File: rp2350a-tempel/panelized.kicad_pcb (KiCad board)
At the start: 2 copper layers, 119.4 x 128.7 mm, 333 parts, among them J1 Conn_North, J2 Conn_East, J3 Conn_South, J4 Conn_West, SW1 BOOT SELECTOR, SW2 RST, U1 AMS1117-3.3, U2 W25Q16JVSS, U3 RP2350_60QFN, Y1 12Mhz HC49-SD

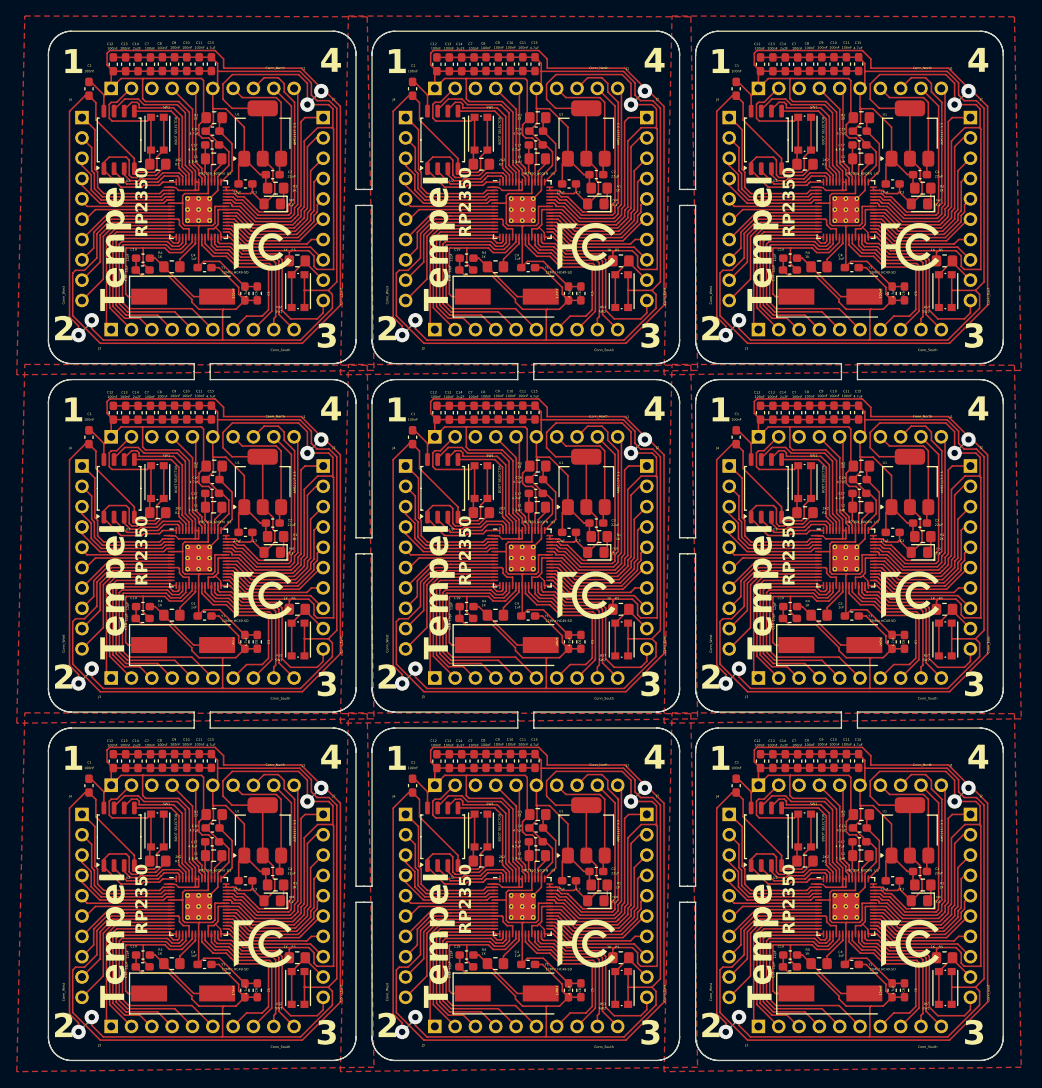
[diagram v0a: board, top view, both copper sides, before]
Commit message: chore: update after first prototype created
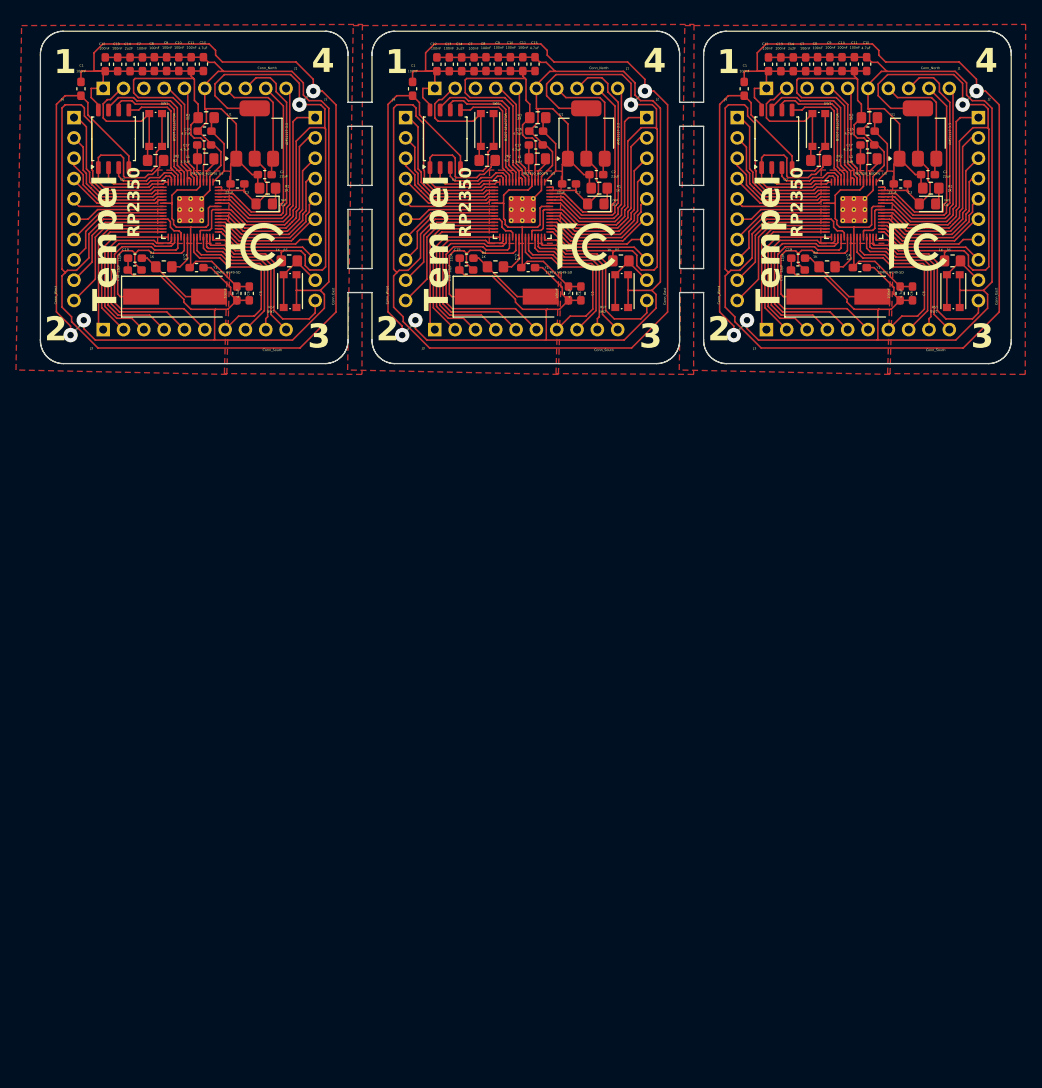
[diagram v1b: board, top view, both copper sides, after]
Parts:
- removed the C1 at (134.3, 70.8)
- removed the C1 at (93.9, 70.8)
- removed the C1 at (174.8, 70.8)
- removed the C1 at (134.3, 114.3)
- removed the C1 at (174.8, 27.2)
- removed the C1 at (93.9, 114.3)
- removed the C1 at (174.8, 114.3)
- removed the C1 at (93.9, 27.2)
- removed the C10 at (187.0, 67.7)
- removed the C10 at (146.6, 111.2)
- removed the C10 at (106.1, 111.2)
- removed the C10 at (146.6, 67.7)
- removed the C10 at (187.0, 111.2)
- removed the C10 at (106.1, 67.7)
- removed the C10 at (106.1, 24.1)
- removed the C10 at (187.0, 24.1)
- removed the C11 at (107.7, 111.2)
- removed the C11 at (188.6, 67.7)
- removed the C11 at (148.1, 111.2)
- removed the C11 at (107.7, 67.7)
- removed the C11 at (188.6, 111.2)
- removed the C11 at (107.7, 24.1)
- removed the C11 at (188.6, 24.1)
- removed the C11 at (148.1, 67.7)
- removed the C12 at (96.9, 111.2)
- removed the C12 at (137.4, 111.2)
- removed the C12 at (96.9, 67.7)
- removed the C12 at (177.8, 24.1)
- removed the C12 at (96.9, 24.1)
- removed the C12 at (177.8, 111.2)
- removed the C12 at (177.8, 67.7)
- removed the C12 at (137.4, 67.7)
- removed the C13 at (138.9, 67.7)
- removed the C13 at (179.4, 67.7)
- removed the C13 at (138.9, 111.2)
- removed the C13 at (98.5, 24.1)
- removed the C13 at (179.4, 111.2)
- removed the C13 at (98.5, 111.2)
- removed the C13 at (179.4, 24.1)
- removed the C13 at (98.5, 67.7)
- removed the C14 at (180.9, 24.1)
- removed the C14 at (180.9, 67.7)
- removed the C14 at (180.9, 111.2)
- removed the C14 at (140.5, 111.2)
- removed the C14 at (100.0, 67.7)
- removed the C14 at (140.5, 67.7)
- removed the C14 at (100.0, 24.1)
- removed the C14 at (100.0, 111.2)
- removed the C15 at (109.2, 111.2)
- removed the C15 at (190.1, 111.2)
- removed the C15 at (109.2, 24.1)
- removed the C15 at (190.1, 67.7)
- removed the C15 at (109.2, 67.7)
- removed the C15 at (149.7, 67.7)
- removed the C15 at (190.1, 24.1)
- removed the C15 at (149.7, 111.2)
- removed the C16 at (109.3, 76.0)
- removed the C16 at (190.2, 32.5)
- removed the C16 at (149.8, 119.6)
- removed the C16 at (190.2, 76.0)
- removed the C16 at (149.8, 76.0)
- removed the C16 at (190.2, 119.6)
- removed the C16 at (109.3, 119.6)
- removed the C16 at (109.3, 32.5)
- removed the C17 at (109.3, 121.3)
- removed the C17 at (149.7, 121.3)
- removed the C17 at (190.2, 77.8)
- removed the C17 at (190.2, 121.3)
- removed the C17 at (109.3, 34.2)
- removed the C17 at (190.2, 34.2)
- removed the C17 at (149.7, 77.8)
- removed the C17 at (109.3, 77.8)
- removed the C18 at (100.6, 137.0)
- removed the C18 at (181.5, 49.8)
- removed the C18 at (181.5, 93.4)
- removed the C18 at (141.1, 93.4)
- removed the C18 at (141.1, 137.0)
- removed the C18 at (100.6, 49.8)
- removed the C18 at (100.6, 93.4)
- removed the C18 at (181.5, 137.0)
- removed the C19 at (141.1, 135.5)
- removed the C19 at (100.6, 91.9)
- removed the C19 at (181.5, 91.9)
- removed the C19 at (100.6, 135.5)
- removed the C19 at (141.1, 91.9)
- removed the C19 at (181.5, 48.4)
- removed the C19 at (181.5, 135.5)
- removed the C19 at (100.6, 48.4)
- removed the C2 at (197.8, 81.5)
- removed the C2 at (157.3, 125.0)
- removed the C2 at (116.9, 81.5)
- removed the C2 at (197.8, 37.9)
- removed the C2 at (197.8, 125.0)
- removed the C2 at (116.9, 125.0)
- removed the C2 at (116.9, 37.9)
- removed the C2 at (157.3, 81.5)
- removed the C3 at (113.5, 39.1)
- removed the C3 at (194.4, 39.1)
- removed the C3 at (113.5, 82.6)
- removed the C3 at (153.9, 82.6)
- removed the C3 at (113.5, 126.2)
- removed the C3 at (194.4, 126.2)
- removed the C3 at (194.4, 82.6)
- removed the C3 at (153.9, 126.2)
- removed the C4 at (189.2, 93.1)
- removed the C4 at (108.3, 136.7)
- removed the C4 at (189.2, 49.5)
- removed the C4 at (148.8, 93.1)
- removed the C4 at (108.3, 49.5)
- removed the C4 at (108.3, 93.1)
- removed the C4 at (189.2, 136.7)
- removed the C4 at (148.8, 136.7)
- removed the C5 at (195.8, 139.9)
- removed the C5 at (195.8, 52.8)
- removed the C5 at (114.9, 96.3)
- removed the C5 at (155.4, 96.3)
- removed the C5 at (114.9, 52.8)
- removed the C5 at (155.4, 139.9)
- removed the C5 at (195.8, 96.3)
- removed the C5 at (114.9, 139.9)
- removed the C6 at (153.8, 96.3)
- removed the C6 at (113.4, 139.9)
- removed the C6 at (194.3, 96.3)
- removed the C6 at (113.4, 52.8)
- removed the C6 at (194.3, 52.8)
- removed the C6 at (113.4, 96.3)
- removed the C6 at (194.3, 139.9)
- removed the C6 at (153.8, 139.9)
- removed the C7 at (182.5, 67.7)
- removed the C7 at (142.0, 67.7)
- removed the C7 at (101.6, 24.1)
- removed the C7 at (182.5, 111.2)
- removed the C7 at (101.6, 111.2)
- removed the C7 at (182.5, 24.1)
- removed the C7 at (101.6, 67.7)
- removed the C7 at (142.0, 111.2)
- removed the C8 at (184.0, 24.1)
- removed the C8 at (103.1, 111.2)
- removed the C8 at (103.1, 24.1)
- removed the C8 at (143.5, 67.7)
- removed the C8 at (184.0, 111.2)
- removed the C8 at (143.5, 111.2)
- removed the C8 at (103.1, 67.7)
- removed the C8 at (184.0, 67.7)
- removed the C9 at (145.1, 111.2)
- removed the C9 at (104.6, 111.2)
- removed the C9 at (185.5, 24.1)
- removed the C9 at (145.1, 67.7)
- removed the C9 at (185.5, 67.7)
- removed the C9 at (104.6, 24.1)
- removed the C9 at (104.6, 67.7)
- removed the C9 at (185.5, 111.2)
- removed the D1 at (116.8, 128.7)
- removed the D1 at (197.7, 128.7)
- removed the D1 at (116.8, 85.1)
- removed the D1 at (197.7, 41.6)
- removed the D1 at (157.3, 128.7)
- removed the D1 at (157.3, 85.1)
- removed the D1 at (197.7, 85.1)
- removed the D1 at (116.8, 41.6)
- removed the J1 at (96.7, 114.3)
- removed the J1 at (137.1, 70.7)
- removed the J1 at (177.6, 114.3)
- removed the J1 at (96.7, 27.1)
- removed the J1 at (177.6, 70.7)
- removed the J1 at (137.1, 114.3)
- removed the J1 at (177.6, 27.1)
- removed the J1 at (96.7, 70.7)
- removed the J2 at (163.6, 117.9)
- removed the J2 at (123.2, 30.8)
- removed the J2 at (163.6, 74.4)
- removed the J2 at (123.2, 117.9)
- removed the J2 at (204.1, 74.4)
- removed the J2 at (123.2, 74.4)
- removed the J2 at (204.1, 117.9)
- removed the J2 at (204.1, 30.8)
- removed the J3 at (96.7, 144.4)
- removed the J3 at (137.1, 100.9)
- removed the J3 at (177.6, 100.9)
- removed the J3 at (177.6, 144.4)
- removed the J3 at (177.6, 57.3)
- removed the J3 at (96.7, 57.3)
- removed the J3 at (96.7, 100.9)
- removed the J3 at (137.1, 144.4)
- removed the J4 at (93.0, 117.9)
- removed the J4 at (93.0, 74.4)
- removed the J4 at (133.5, 117.9)
- removed the J4 at (93.0, 30.8)
- removed the J4 at (173.9, 117.9)
- removed the J4 at (133.5, 74.4)
- removed the J4 at (173.9, 30.8)
- removed the J4 at (173.9, 74.4)
- removed the L1 at (109.5, 35.9)
- removed the L1 at (109.5, 123.1)
- removed the L1 at (149.9, 123.1)
- removed the L1 at (109.5, 79.5)
- removed the L1 at (190.4, 79.5)
- removed the L1 at (190.4, 35.9)
- removed the L1 at (190.4, 123.1)
- removed the L1 at (149.9, 79.5)
- removed the R1 at (198.1, 39.6)
- removed the R1 at (157.7, 83.2)
- removed the R1 at (117.2, 126.7)
- removed the R1 at (198.1, 83.2)
- removed the R1 at (117.2, 39.6)
- removed the R1 at (117.2, 83.2)
- removed the R1 at (198.1, 126.7)
- removed the R1 at (157.7, 126.7)
- removed the R2 at (102.5, 80.2)
- removed the R2 at (183.4, 80.2)
- removed the R2 at (142.9, 80.2)
- removed the R2 at (183.4, 123.7)
- removed the R2 at (142.9, 123.7)
- removed the R2 at (142.9, 36.6)
- removed the R2 at (102.5, 36.6)
- removed the R2 at (183.4, 36.6)
- removed the R2 at (102.5, 123.7)
- removed the R3 at (109.5, 74.4)
- removed the R3 at (109.5, 117.9)
- removed the R3 at (109.5, 30.8)
- removed the R3 at (190.4, 117.9)
- removed the R3 at (150.0, 74.4)
- removed the R3 at (190.4, 74.4)
- removed the R3 at (190.4, 30.8)
- removed the R3 at (150.0, 117.9)
- removed the R4 at (104.3, 49.4)
- removed the R4 at (185.2, 49.4)
- removed the R4 at (185.2, 136.6)
- removed the R4 at (144.7, 93.0)
- removed the R4 at (144.7, 136.6)
- removed the R4 at (185.2, 93.0)
- removed the R4 at (104.3, 136.6)
- removed the R4 at (104.3, 93.0)
- removed the R5 at (200.8, 135.8)
- removed the R5 at (119.9, 135.8)
- removed the R5 at (119.9, 48.7)
- removed the R5 at (119.9, 92.3)
- removed the R5 at (200.8, 48.7)
- removed the R5 at (160.4, 92.3)
- removed the R5 at (200.8, 92.3)
- removed the R5 at (160.4, 135.8)
- removed the REF** at (115.6, 134.1)
- removed the REF** at (196.5, 134.1)
- removed the REF** at (196.5, 90.5)
- removed the REF** at (156.1, 90.5)
- removed the REF** at (196.5, 46.9)
- removed the REF** at (115.6, 46.9)
- removed the REF** at (115.6, 90.5)
- removed the REF** at (156.1, 134.1)
- removed the SW1 at (183.3, 76.4)
- removed the SW1 at (183.3, 32.8)
- removed the SW1 at (142.9, 76.4)
- removed the SW1 at (142.9, 32.8)
- removed the SW1 at (102.4, 32.8)
- removed the SW1 at (102.4, 119.9)
- removed the SW1 at (142.9, 119.9)
- removed the SW1 at (102.4, 76.4)
- removed the SW1 at (183.3, 119.9)
- removed the SW2 at (200.9, 96.0)
- removed the SW2 at (200.9, 52.5)
- removed the SW2 at (120.0, 96.0)
- removed the SW2 at (120.0, 52.5)
- removed the SW2 at (160.5, 96.0)
- removed the SW2 at (200.9, 139.6)
- removed the SW2 at (120.0, 139.6)
- removed the SW2 at (160.5, 139.6)
- removed the U1 at (196.5, 119.9)
- removed the U1 at (156.1, 76.3)
- removed the U1 at (196.5, 76.3)
- removed the U1 at (115.6, 119.9)
- removed the U1 at (156.1, 119.9)
- removed the U1 at (115.6, 76.3)
- removed the U1 at (115.6, 32.8)
- removed the U1 at (196.5, 32.8)
- removed the U2 at (178.6, 120.7)
- removed the U2 at (138.1, 33.6)
- removed the U2 at (178.6, 33.6)
- removed the U2 at (97.7, 33.6)
- removed the U2 at (138.1, 120.7)
- removed the U2 at (138.1, 77.1)
- removed the U2 at (178.6, 77.1)
- removed the U2 at (97.7, 120.7)
- removed the U2 at (97.7, 77.1)
- removed the U3 at (188.5, 129.4)
- removed the U3 at (148.1, 85.9)
- removed the U3 at (148.1, 129.4)
- removed the U3 at (107.6, 85.9)
- removed the U3 at (107.6, 42.3)
- removed the U3 at (107.6, 129.4)
- removed the U3 at (188.5, 85.9)
- removed the U3 at (188.5, 42.3)
- removed the Y1 at (105.7, 140.3)
- removed the Y1 at (146.1, 96.7)
- removed the Y1 at (186.6, 53.2)
- removed the Y1 at (186.6, 140.3)
- removed the Y1 at (105.7, 96.7)
- removed the Y1 at (146.1, 140.3)
- removed the Y1 at (105.7, 53.2)
- removed the Y1 at (186.6, 96.7)
- added C1: 100nF, Capacitor_SMD:C_0603_1608Metric_Pad1.08x0.95mm_HandSolder, F.Cu at (92.9, 27.2)
- added C1: 100nF, Capacitor_SMD:C_0603_1608Metric_Pad1.08x0.95mm_HandSolder, F.Cu at (175.8, 27.2)
- added C10: 100nF, Capacitor_SMD:C_0603_1608Metric_Pad1.08x0.95mm_HandSolder, F.Cu at (105.1, 24.1)
- added C10: 100nF, Capacitor_SMD:C_0603_1608Metric_Pad1.08x0.95mm_HandSolder, F.Cu at (188.0, 24.1)
- added C11: 100nF, Capacitor_SMD:C_0603_1608Metric_Pad1.08x0.95mm_HandSolder, F.Cu at (106.7, 24.1)
- added C11: 100nF, Capacitor_SMD:C_0603_1608Metric_Pad1.08x0.95mm_HandSolder, F.Cu at (189.6, 24.1)
- added C12: 100nF, Capacitor_SMD:C_0603_1608Metric_Pad1.08x0.95mm_HandSolder, F.Cu at (178.8, 24.1)
- added C12: 100nF, Capacitor_SMD:C_0603_1608Metric_Pad1.08x0.95mm_HandSolder, F.Cu at (95.9, 24.1)
- added C13: 100nF, Capacitor_SMD:C_0603_1608Metric_Pad1.08x0.95mm_HandSolder, F.Cu at (180.4, 24.1)
- added C13: 100nF, Capacitor_SMD:C_0603_1608Metric_Pad1.08x0.95mm_HandSolder, F.Cu at (97.5, 24.1)
- added C14: 2u2F, Capacitor_SMD:C_0603_1608Metric_Pad1.08x0.95mm_HandSolder, F.Cu at (181.9, 24.1)
- added C14: 2u2F, Capacitor_SMD:C_0603_1608Metric_Pad1.08x0.95mm_HandSolder, F.Cu at (99.0, 24.1)
- added C15: 4.7uF, Capacitor_SMD:C_0603_1608Metric_Pad1.08x0.95mm_HandSolder, F.Cu at (191.1, 24.1)
- added C15: 4.7uF, Capacitor_SMD:C_0603_1608Metric_Pad1.08x0.95mm_HandSolder, F.Cu at (108.2, 24.1)
- added C16: 4.7uF, Capacitor_SMD:C_0603_1608Metric_Pad1.08x0.95mm_HandSolder, F.Cu at (108.3, 32.5)
- added C16: 4.7uF, Capacitor_SMD:C_0603_1608Metric_Pad1.08x0.95mm_HandSolder, F.Cu at (191.2, 32.5)
- added C17: 4.7uF, Capacitor_SMD:C_0603_1608Metric_Pad1.08x0.95mm_HandSolder, F.Cu at (191.2, 34.2)
- added C17: 4.7uF, Capacitor_SMD:C_0603_1608Metric_Pad1.08x0.95mm_HandSolder, F.Cu at (108.3, 34.2)
- added C18: 12pF, Capacitor_SMD:C_0603_1608Metric_Pad1.08x0.95mm_HandSolder, F.Cu at (182.5, 49.8)
- added C18: 12pF, Capacitor_SMD:C_0603_1608Metric_Pad1.08x0.95mm_HandSolder, F.Cu at (99.6, 49.8)
- added C19: 12pF, Capacitor_SMD:C_0603_1608Metric_Pad1.08x0.95mm_HandSolder, F.Cu at (99.6, 48.4)
- added C19: 12pF, Capacitor_SMD:C_0603_1608Metric_Pad1.08x0.95mm_HandSolder, F.Cu at (182.5, 48.4)
- added C2: 22uF, Capacitor_SMD:C_0603_1608Metric_Pad1.08x0.95mm_HandSolder, F.Cu at (115.9, 37.9)
- added C2: 22uF, Capacitor_SMD:C_0603_1608Metric_Pad1.08x0.95mm_HandSolder, F.Cu at (198.8, 37.9)
- added C3: 22uF, Capacitor_SMD:C_0603_1608Metric_Pad1.08x0.95mm_HandSolder, F.Cu at (195.4, 39.1)
- added C3: 22uF, Capacitor_SMD:C_0603_1608Metric_Pad1.08x0.95mm_HandSolder, F.Cu at (112.5, 39.1)
- added C4: 1uF, Capacitor_SMD:C_0603_1608Metric_Pad1.08x0.95mm_HandSolder, F.Cu at (107.3, 49.5)
- added C4: 1uF, Capacitor_SMD:C_0603_1608Metric_Pad1.08x0.95mm_HandSolder, F.Cu at (190.2, 49.5)
- added C5: 4.7uF, Capacitor_SMD:C_0603_1608Metric_Pad1.08x0.95mm_HandSolder, F.Cu at (113.9, 52.8)
- added C5: 4.7uF, Capacitor_SMD:C_0603_1608Metric_Pad1.08x0.95mm_HandSolder, F.Cu at (196.8, 52.8)
- added C6: 100nF, Capacitor_SMD:C_0603_1608Metric_Pad1.08x0.95mm_HandSolder, F.Cu at (112.4, 52.8)
- added C6: 100nF, Capacitor_SMD:C_0603_1608Metric_Pad1.08x0.95mm_HandSolder, F.Cu at (195.3, 52.8)
- added C7: 100nF, Capacitor_SMD:C_0603_1608Metric_Pad1.08x0.95mm_HandSolder, F.Cu at (183.5, 24.1)
- added C7: 100nF, Capacitor_SMD:C_0603_1608Metric_Pad1.08x0.95mm_HandSolder, F.Cu at (100.6, 24.1)
- added C8: 100nF, Capacitor_SMD:C_0603_1608Metric_Pad1.08x0.95mm_HandSolder, F.Cu at (185.0, 24.1)
- added C8: 100nF, Capacitor_SMD:C_0603_1608Metric_Pad1.08x0.95mm_HandSolder, F.Cu at (102.1, 24.1)
- added C9: 100nF, Capacitor_SMD:C_0603_1608Metric_Pad1.08x0.95mm_HandSolder, F.Cu at (186.5, 24.1)
- added C9: 100nF, Capacitor_SMD:C_0603_1608Metric_Pad1.08x0.95mm_HandSolder, F.Cu at (103.6, 24.1)
- added D1: red, LED_SMD:LED_0805_2012Metric_Pad1.15x1.40mm_HandSolder, F.Cu at (115.8, 41.6)
- added D1: red, LED_SMD:LED_0805_2012Metric_Pad1.15x1.40mm_HandSolder, F.Cu at (198.7, 41.6)
- added J1: Conn_North, Connector_PinHeader_2.54mm:PinHeader_1x10_P2.54mm_Vertical, B.Cu at (178.6, 27.1)
- added J1: Conn_North, Connector_PinHeader_2.54mm:PinHeader_1x10_P2.54mm_Vertical, B.Cu at (95.7, 27.1)
- added J2: Conn_East, Connector_PinHeader_2.54mm:PinHeader_1x10_P2.54mm_Vertical, B.Cu at (205.1, 30.8)
- added J2: Conn_East, Connector_PinHeader_2.54mm:PinHeader_1x10_P2.54mm_Vertical, B.Cu at (122.2, 30.8)
- added J3: Conn_South, Connector_PinHeader_2.54mm:PinHeader_1x10_P2.54mm_Vertical, B.Cu at (178.6, 57.3)
- added J3: Conn_South, Connector_PinHeader_2.54mm:PinHeader_1x10_P2.54mm_Vertical, B.Cu at (95.7, 57.3)
- added J4: Conn_West, Connector_PinHeader_2.54mm:PinHeader_1x10_P2.54mm_Vertical, B.Cu at (174.9, 30.8)
- added J4: Conn_West, Connector_PinHeader_2.54mm:PinHeader_1x10_P2.54mm_Vertical, B.Cu at (92.0, 30.8)
- added L1: 3.3uH, Inductor_SMD:L_0805_2012Metric_Pad1.15x1.40mm_HandSolder, F.Cu at (108.5, 35.9)
- added L1: 3.3uH, Inductor_SMD:L_0805_2012Metric_Pad1.15x1.40mm_HandSolder, F.Cu at (191.4, 35.9)
- added R1: 1K, Resistor_SMD:R_0805_2012Metric_Pad1.20x1.40mm_HandSolder, F.Cu at (199.1, 39.6)
- added R1: 1K, Resistor_SMD:R_0805_2012Metric_Pad1.20x1.40mm_HandSolder, F.Cu at (116.2, 39.6)
- added R2: 2K2, Resistor_SMD:R_0805_2012Metric_Pad1.20x1.40mm_HandSolder, F.Cu at (143.7, 36.1)
- added R2: 2K2, Resistor_SMD:R_0805_2012Metric_Pad1.20x1.40mm_HandSolder, F.Cu at (102.2, 36.1)
- added R2: 2K2, Resistor_SMD:R_0805_2012Metric_Pad1.20x1.40mm_HandSolder, F.Cu at (185.1, 36.1)
- added R3: 33, Resistor_SMD:R_0805_2012Metric_Pad1.20x1.40mm_HandSolder, F.Cu at (191.4, 30.8)
- added R3: 33, Resistor_SMD:R_0805_2012Metric_Pad1.20x1.40mm_HandSolder, F.Cu at (108.5, 30.8)
- added R4: 1K, Resistor_SMD:R_0805_2012Metric_Pad1.20x1.40mm_HandSolder, F.Cu at (103.3, 49.4)
- added R4: 1K, Resistor_SMD:R_0805_2012Metric_Pad1.20x1.40mm_HandSolder, F.Cu at (186.2, 49.4)
- added R5: 1K, Resistor_SMD:R_0805_2012Metric_Pad1.20x1.40mm_HandSolder, F.Cu at (118.9, 48.7)
- added R5: 1K, Resistor_SMD:R_0805_2012Metric_Pad1.20x1.40mm_HandSolder, F.Cu at (201.8, 48.7)
- added REF**: FCC-Logo_7.3x6mm_SilkScreen, Symbol:FCC-Logo_7.3x6mm_SilkScreen, F.Cu at (114.6, 46.9)
- added REF**: FCC-Logo_7.3x6mm_SilkScreen, Symbol:FCC-Logo_7.3x6mm_SilkScreen, F.Cu at (197.5, 46.9)
- added SW1: BOOT SELECTOR, Button_Switch_SMD:SW_Push_1P1T_NO_CK_KMR2, F.Cu at (143.7, 32.3)
- added SW1: BOOT SELECTOR, Button_Switch_SMD:SW_Push_1P1T_NO_CK_KMR2, F.Cu at (102.2, 32.3)
- added SW1: BOOT SELECTOR, Button_Switch_SMD:SW_Push_1P1T_NO_CK_KMR2, F.Cu at (185.1, 32.3)
- added SW2: RST, Button_Switch_SMD:SW_Push_1P1T_NO_CK_KMR2, F.Cu at (201.9, 52.5)
- added SW2: RST, Button_Switch_SMD:SW_Push_1P1T_NO_CK_KMR2, F.Cu at (119.0, 52.5)
- added U1: AMS1117-3.3, Package_TO_SOT_SMD:SOT-223-3_TabPin2, F.Cu at (197.5, 32.8)
- added U1: AMS1117-3.3, Package_TO_SOT_SMD:SOT-223-3_TabPin2, F.Cu at (114.6, 32.8)
- added U2: W25Q16JVSS, Package_SO:SOIC-8_5.23x5.23mm_P1.27mm, F.Cu at (97.0, 33.4)
- added U2: W25Q16JVSS, Package_SO:SOIC-8_5.23x5.23mm_P1.27mm, F.Cu at (138.4, 33.4)
- added U2: W25Q16JVSS, Package_SO:SOIC-8_5.23x5.23mm_P1.27mm, F.Cu at (179.9, 33.4)
- added U3: RP2350_60QFN, lib:RP2350-QFN-60-1EP_7x7_P0.4mm_EP3.4x3.4mm_ThermalVias, F.Cu at (106.6, 42.3)
- added U3: RP2350_60QFN, lib:RP2350-QFN-60-1EP_7x7_P0.4mm_EP3.4x3.4mm_ThermalVias, F.Cu at (189.5, 42.3)
- added Y1: 12Mhz HC49-SD, Crystal:Crystal_SMD_HC49-SD, F.Cu at (104.7, 53.2)
- added Y1: 12Mhz HC49-SD, Crystal:Crystal_SMD_HC49-SD, F.Cu at (187.6, 53.2)
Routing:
- net Board_7-+3.3V: track 313.0 -> 0.00 mm, vias 2 -> 0
- net Board_8-+3.3V: track 313.0 -> 0.00 mm, vias 2 -> 0
- net Board_5-+3.3V: track 313.0 -> 0.00 mm, vias 2 -> 0
- net Board_4-+3.3V: track 313.0 -> 0.00 mm, vias 2 -> 0
- net Board_6-+3.3V: track 313.0 -> 0.00 mm, vias 2 -> 0
- net Board_3-+3.3V: track 313.0 -> 0.00 mm, vias 2 -> 0
- net Board_4-GND: track 220.9 -> 0.00 mm, vias 2 -> 0
- net Board_3-GND: track 220.9 -> 0.00 mm, vias 2 -> 0
- net Board_7-GND: track 220.9 -> 0.00 mm, vias 2 -> 0
- net Board_6-GND: track 220.9 -> 0.00 mm, vias 2 -> 0
- net Board_5-GND: track 220.9 -> 0.00 mm, vias 2 -> 0
- net Board_8-GND: track 220.9 -> 0.00 mm, vias 2 -> 0
- net Board_1-+3.3V: track 313.0 -> 353.5 mm
- net Board_2-+3.3V: track 313.0 -> 353.5 mm
- net Board_0-+3.3V: track 313.0 -> 353.5 mm
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- removed copper zone on F.Cu, net Board_3-+3.3V
- removed copper zone on F.Cu, net Board_4-+3.3V
- removed copper zone on F.Cu, net Board_5-+3.3V
- removed copper zone on F.Cu, net Board_6-+3.3V
- removed copper zone on F.Cu, net Board_7-+3.3V
- removed copper zone on F.Cu, net Board_8-+3.3V
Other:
- board size 119.4 x 128.7 mm -> 121.4 x 41.6 mm
